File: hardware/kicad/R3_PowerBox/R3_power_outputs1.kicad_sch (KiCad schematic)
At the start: 7 parts, among them J10 BATTERY / CHARGER TELEMETRY, J2 DIGITAL POWER OUT, J3 ISOLATED POWER OUT, J4 CONTROL / SERVICE, J5 PRIMARY AUX DNP, J6 ISOLATED AUX DNP

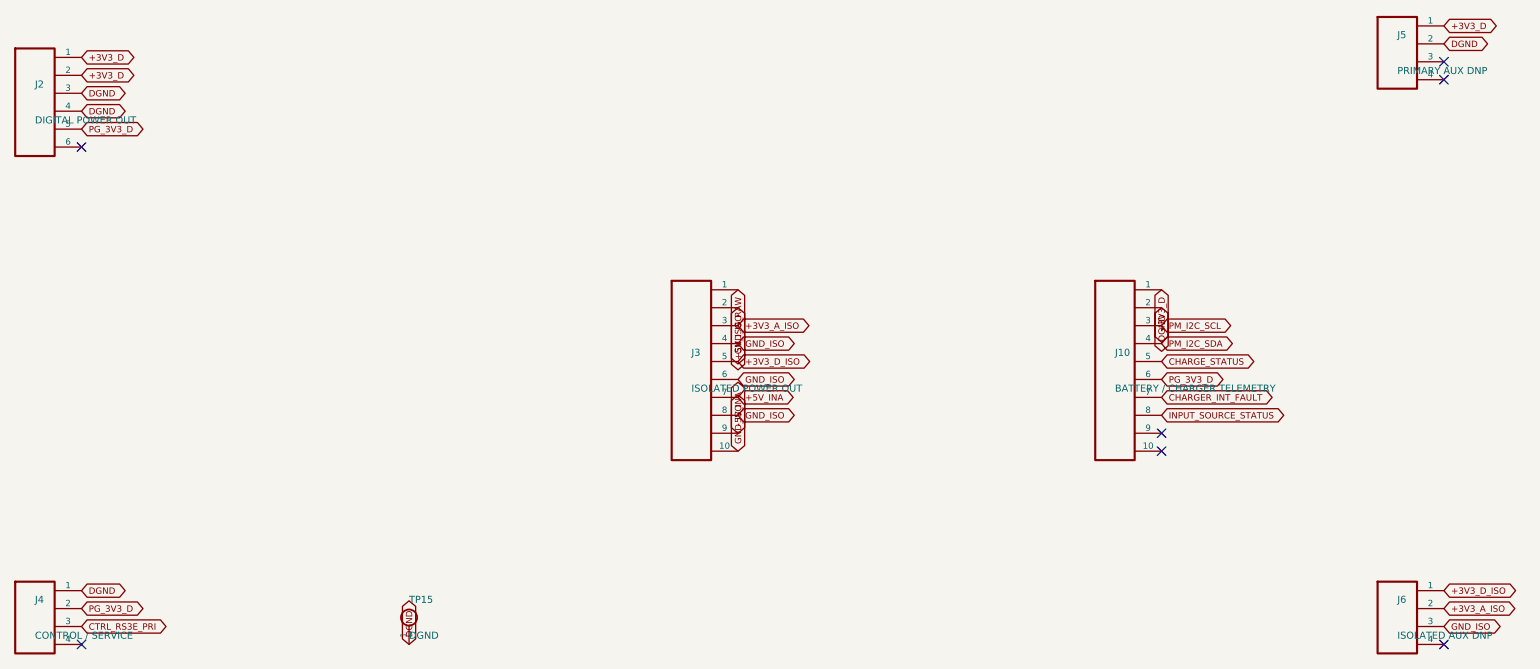
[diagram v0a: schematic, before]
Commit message: Finalize R3 PowerBox pre-placement corrections
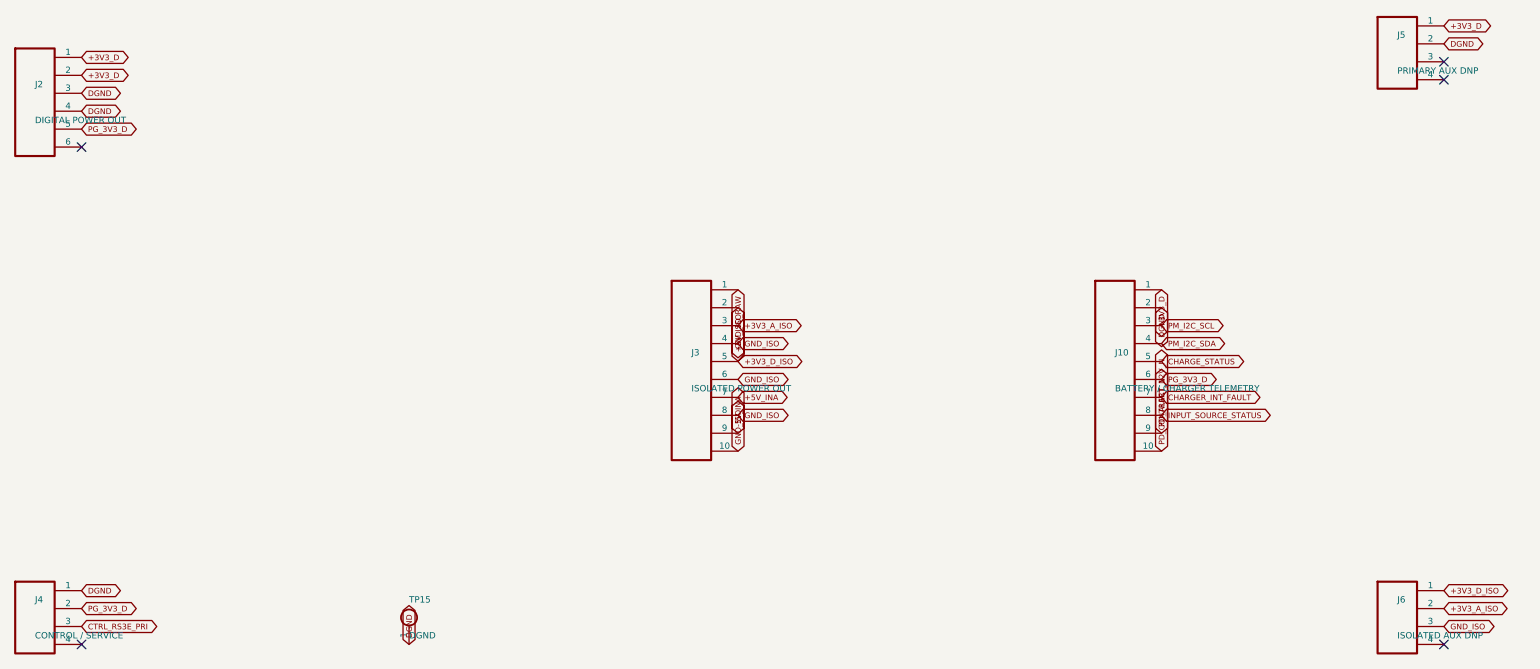
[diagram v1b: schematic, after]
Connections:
- net PD_CONTRACT_12V_N: now reaches J10.10
- net PD_ALERT_N: now reaches J10.9
- no-connect marks 7 -> 5
